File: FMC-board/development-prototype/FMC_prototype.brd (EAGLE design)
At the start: 103.8 x 69.8 mm, 69 parts, among them J1 DC_POWER_JACK-PJ-102AH, J2 DC_POWER_JACK-PJ-102AH

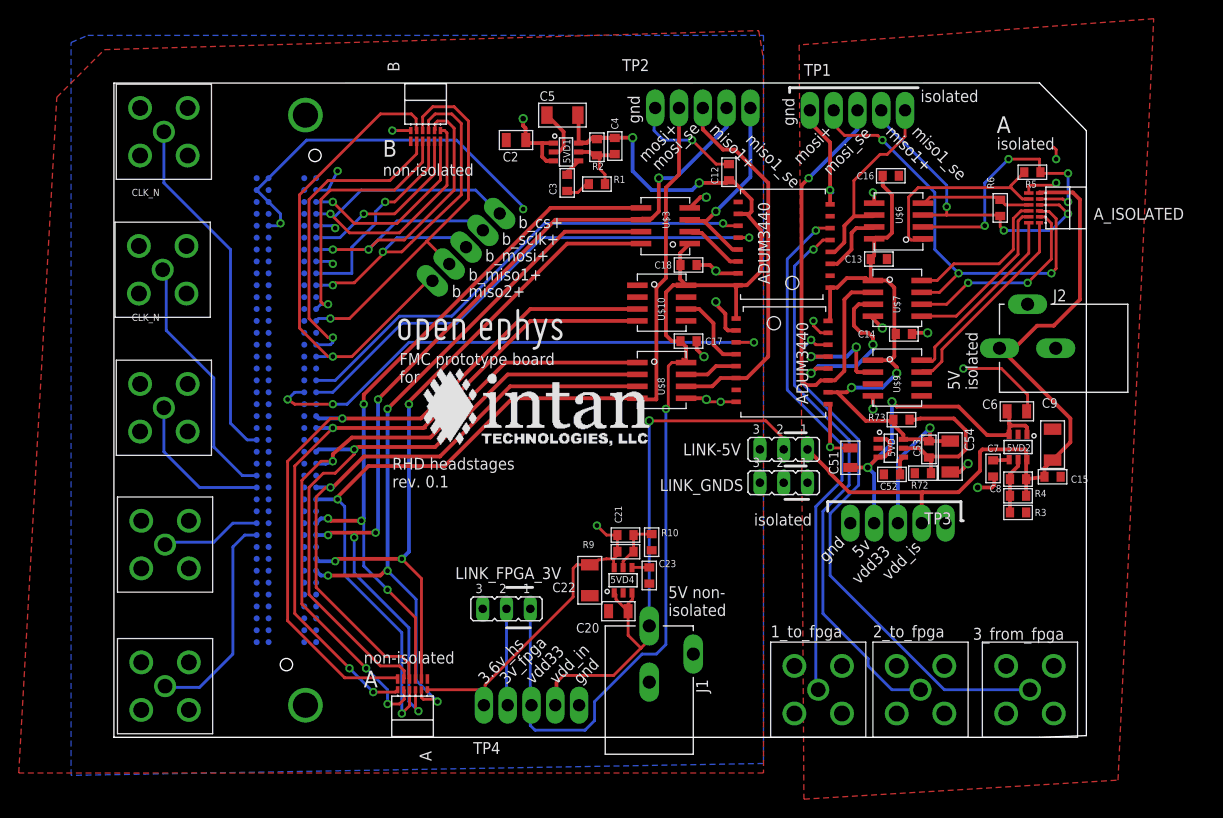
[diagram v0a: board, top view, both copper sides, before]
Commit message: cleanup, starting DRC
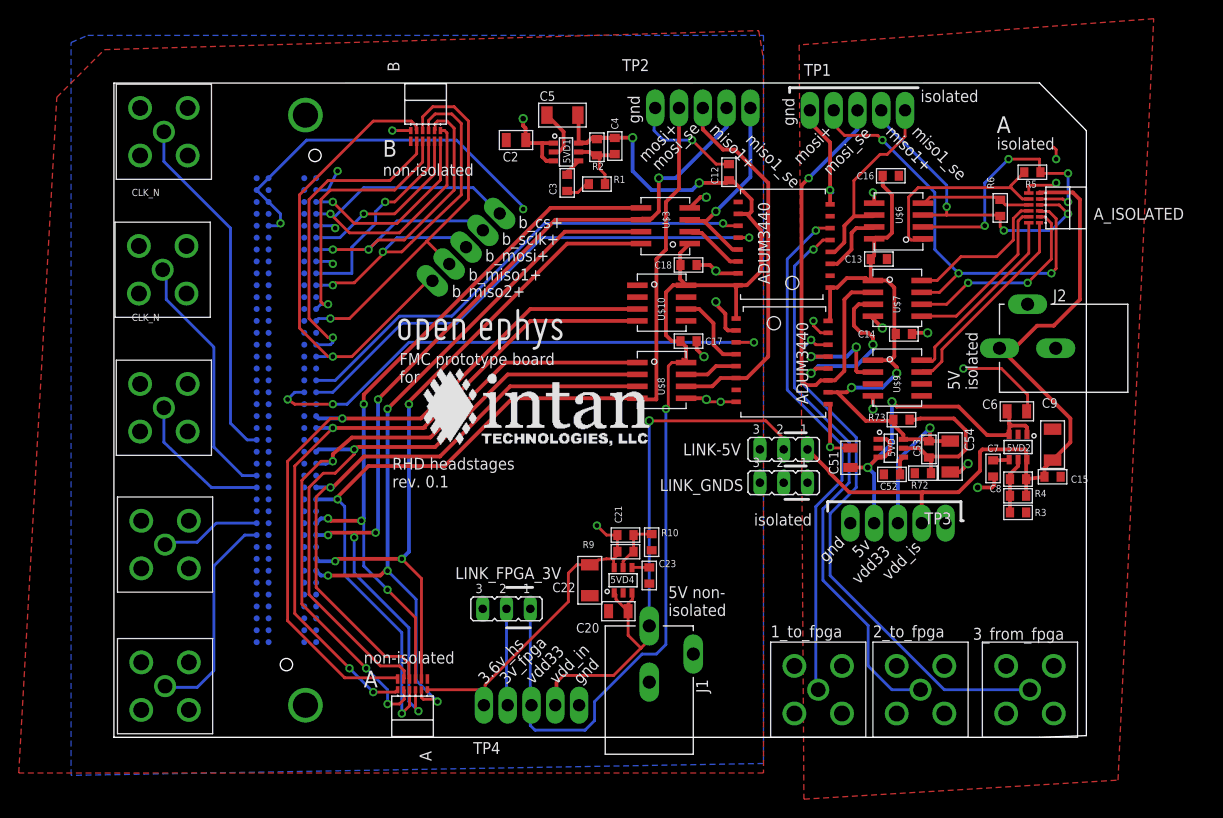
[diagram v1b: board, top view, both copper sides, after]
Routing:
- net B_MISO2+: track 52.3 -> 51.3 mm
- net TP6: track 16.2 -> 15.5 mm
- net MOSI-_ISOLATED: track 16.4 -> 15.9 mm
